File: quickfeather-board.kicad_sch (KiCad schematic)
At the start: 101 parts, among them IC1 EOSAI-S-PUN64, J1 PinHeader_1x2_P2.54mm_Drill1.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, J2 PinHeader_1x12_P2.54m_Drill1.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, J3 61301611121, J4 S2B-PH-SM4-TB(LF)(SN), J5 USB-Micro-B_Molex_473460001, J6 PinHeader_2x5_P1.27mm_SMD_Lat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, J7 PinHeader_1x2_P2.54mm_Drill1.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, J8 PinHeader_2x8_P2.54mm_Drill1mm, Q1 NX3008CBKV, Q2 2N7002PV, Q3 2N7002PV, Q4 DMG1012T-7, U1 TPS62821DLCR, U2 MCP73831T-2AC_SOT, U3 GD25Q16CWIGR, U4 DPS310, U5 MC3635, X1 Resonator_12MHz_445

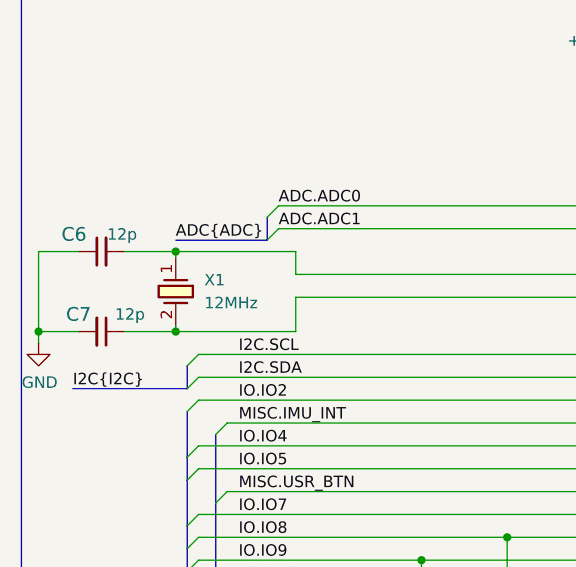
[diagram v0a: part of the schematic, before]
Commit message: [#54927] Update X1
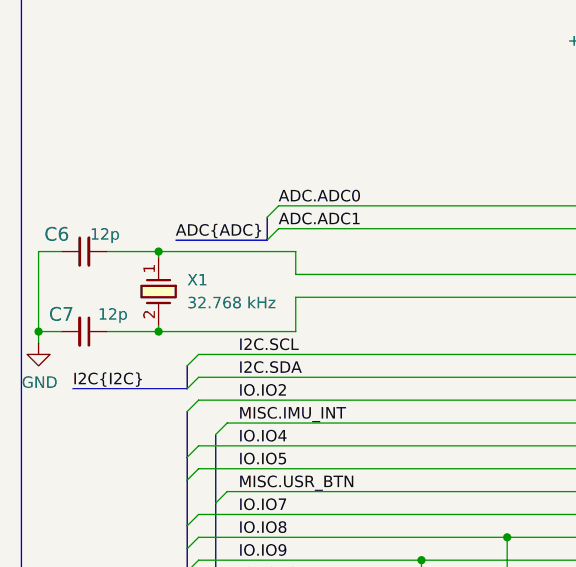
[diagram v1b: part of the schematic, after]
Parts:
- X1: value Resonator_12MHz_445 -> Resonator_32.768kHz_ECX-31B; footprint antmicro-footprints:Resonator_SMD_CTS_445_5x3.2mm -> antmicro-footprints:SMD-2_3.2x1.5mm; symbol antmicroResonators:Resonator_12MHz_445 -> antmicroResonators:Resonator_32.768kHz_ECX-31B; MPN 445I23D12M00000 -> ECS-.327-12.5-34B-TR; Manufacturer CTS -> ECS Inc. International; Val 12MHz -> 32.768 kHz
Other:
- moved on the sheet: C6, C7, X1
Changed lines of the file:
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@@
   (junction (at 356.87 130.81) (diameter 0) (color 0 0 0 0)
   )
+  (junction (at 29.21 44.45) (diameter 0) (color 0 0 0 0)
+  )
   (junction (at 396.875 172.085) (diameter 0) (color 0 0 0 0)
   )
@@
   (junction (at 328.93 34.29) (diameter 0) (color 0 0 0 0)
   )
-  (junction (at 31.115 53.34) (diameter 0) (color 0 0 0 0)
-  )
   (junction (at 76.2 124.46) (diameter 0) (color 0 0 0 0)
   )
+  (junction (at 29.21 53.34) (diameter 0) (color 0 0 0 0)
+  )
   (junction (at 15.875 53.34) (diameter 0) (color 0 0 0 0)
   )
@@
   (junction (at 52.705 220.98) (diameter 0) (color 0 0 0 0)
   )
-  (junction (at 31.115 44.45) (diameter 0) (color 0 0 0 0)
-  )
   (junction (at 194.945 158.115) (diameter 0) (color 0 0 0 0)
   )
@@
     (stroke (width 0) (type default))
   )
-  (wire (pts (xy 25.4 53.34) (xy 31.115 53.34))
+  (wire (pts (xy 23.495 53.34) (xy 29.21 53.34))
     (stroke (width 0) (type default))
   )
@@
     (stroke (width 0) (type default))
   )
+  (wire (pts (xy 29.21 53.34) (xy 44.45 53.34))
+    (stroke (width 0) (type default))
+  )
   (wire (pts (xy 178.435 156.21) (xy 178.435 162.56))
     (stroke (width 0) (type default))
@@
     (stroke (width 0) (type default))
   )
-  (wire (pts (xy 15.875 53.34) (xy 20.32 53.34))
+  (wire (pts (xy 15.875 53.34) (xy 18.415 53.34))
     (stroke (width 0) (type default))
   )
@@
     (stroke (width 0) (type default))
   )
-  (wire (pts (xy 15.875 44.45) (xy 20.32 44.45))
+  (wire (pts (xy 15.875 44.45) (xy 18.415 44.45))
     (stroke (width 0) (type default))
   )
@@
     (stroke (width 0) (type default))
   )
-  (wire (pts (xy 31.115 44.45) (xy 44.45 44.45))
+  (wire (pts (xy 29.21 44.45) (xy 44.45 44.45))
     (stroke (width 0) (type default))
   )
@@
     (stroke (width 0) (type default))
   )
-  (wire (pts (xy 25.4 44.45) (xy 31.115 44.45))
+  (wire (pts (xy 23.495 44.45) (xy 29.21 44.45))
     (stroke (width 0) (type default))
   )
@@
     (stroke (width 0) (type default))
   )
-  (wire (pts (xy 31.115 53.34) (xy 31.115 52.705))
+  (wire (pts (xy 29.21 53.34) (xy 29.21 52.705))
     (stroke (width 0) (type default))
   )
@@
     (stroke (width 0) (type default))
   )
-  (wire (pts (xy 31.115 45.085) (xy 31.115 44.45))
+  (wire (pts (xy 29.21 45.085) (xy 29.21 44.45))
     (stroke (width 0) (type default))
   )
@@
     (stroke (width 0) (type default))
   )
-  (wire (pts (xy 44.45 53.34) (xy 31.115 53.34))
-    (stroke (width 0) (type default))
-  )
   (wire (pts (xy 234.315 221.615) (xy 234.315 231.14))
     (stroke (width 0) (type default))
@@
     )
   )
-  (symbol (lib_id "antmicroResonators:Resonator_12MHz_445") (at 31.115 45.085 270) (unit 1)
+  (symbol (lib_id "antmicroResonators:Resonator_32.768kHz_ECX-31B") (at 29.21 45.085 270) (unit 1)
     (in_bom yes) (on_board yes) (dnp no) (fields_autoplaced)
-    (property "Reference" "X1" (at 34.29 47.625 90)
+    (property "Reference" "X1" (at 32.385 47.625 90)
       (effects (font (size 1.27 1.27)) (justify left))
     )
-    (property "Value" "Resonator_12MHz_445" (at 15.875 60.325 0)
+    (property "Value" "Resonator_32.768kHz_ECX-31B" (at 13.97 60.325 0)
       (effects (font (size 1.27 1.27) (thickness 0.15)) (justify left bottom) hide)
     )
-    (property "Footprint" "antmicro-footprints:Resonator_SMD_CTS_445_5x3.2mm" (at 13.335 60.325 0)
+    (property "Footprint" "antmicro-footprints:SMD-2_3.2x1.5mm" (at 11.43 60.325 0)
       (effects (font (size 1.27 1.27) (thickness 0.15)) (justify left bottom) hide)
     )
-    (property "Datasheet" "https://www.ctscorp.com/wp-content/uploads/445.pdf" (at 10.795 60.325 0)
+    (property "Datasheet" "http://www.ecsxtal.com/store/pdf/ecx-31b.pdf" (at 8.89 60.325 0)
       (effects (font (size 1.27 1.27) (thickness 0.15)) (justify left bottom) hide)
     )
-    (property "MPN" "445I23D12M00000" (at 34.925 48.895 90)
-      (effects (font (size 1.27 1.27) (thickness 0.15)) (justify left) hide)
+    (property "MPN" "ECS-.327-12.5-34B-TR" (at 21.59 60.325 0)
+      (effects (font (size 1.27 1.27) (thickness 0.15)) (justify left bottom) hide)
     )
-    (property "Manufacturer" "CTS" (at 20.955 60.325 0)
+    (property "Manufacturer" "ECS Inc. International" (at 19.05 60.325 0)
       (effects (font (size 1.27 1.27) (thickness 0.15)) (justify left bottom) hide)
     )
-    (property "Val" "12MHz" (at 34.29 50.165 90)
+    (property "Val" "32.768 kHz" (at 32.385 50.165 90)
       (effects (font (size 1.27 1.27) (thickness 0.15)) (justify left))
     )
-    (property "Author" "Antmicro" (at 8.255 60.325 0)
+    (property "Author" "Antmicro" (at 6.35 60.325 0)
       (effects (font (size 1.27 1.27) (thickness 0.15)) (justify left bottom) hide)
     )
-    (property "License" "Apache-2.0" (at 5.715 60.325 0)
+    (property "License" "Apache-2.0" (at 3.81 60.325 0)
       (effects (font (size 1.27 1.27) (thickness 0.15)) (justify left bottom) hide)
     )
@@
     )
   )
-  (symbol (lib_id "antmicroCapacitors0402:C_12p_0402") (at 20.32 44.45 0) (unit 1)
+  (symbol (lib_id "antmicroCapacitors0402:C_12p_0402") (at 18.415 44.45 0) (unit 1)
     (in_bom yes) (on_board yes) (dnp no)
-    (property "Reference" "C6" (at 18.415 42.545 0)
+    (property "Reference" "C6" (at 16.51 42.545 0)
       (effects (font (size 1.524 1.524)) (justify left))
     )
-    (property "Value" "C_12p_0402" (at 20.32 48.26 0)
+    (property "Value" "C_12p_0402" (at 18.415 48.26 0)
       (effects (font (size 1.524 1.524)) hide)
     )
-    (property "Footprint" "antmicro-footprints:C_0402_1005Metric" (at 25.4 39.37 0)
+    (property "Footprint" "antmicro-footprints:C_0402_1005Metric" (at 23.495 39.37 0)
       (effects (font (size 1.524 1.524)) (justify left) hide)
     )
-    (property "Datasheet" "https://product.tdk.com/en/search/capacitor/ceramic/mlcc/info?part_no=CGA2B2C0G1H120J050BA" (at 20.32 44.45 0)
+    (property "Datasheet" "https://product.tdk.com/en/search/capacitor/ceramic/mlcc/info?part_no=CGA2B2C0G1H120J050BA" (at 18.415 44.45 0)
       (effects (font (size 1.27 1.27)) hide)
     )
-    (property "Manufacturer" "TDK" (at 25.4 34.29 0)
+    (property "Manufacturer" "TDK" (at 23.495 34.29 0)
       (effects (font (size 1.524 1.524)) (justify left) hide)
     )
-    (property "MPN" "CGA2B2C0G1H120J050BA" (at 25.4 36.83 0)
+    (property "MPN" "CGA2B2C0G1H120J050BA" (at 23.495 36.83 0)
       (effects (font (size 1.524 1.524)) (justify left) hide)
     )
-    (property "Val" "12p" (at 23.495 42.545 0)
+    (property "Val" "12p" (at 21.59 42.545 0)
       (effects (font (size 1.27 1.27)) (justify left))
     )
-    (property "License" "Apache-2.0" (at 40.64 67.31 0)
+    (property "License" "Apache-2.0" (at 38.735 67.31 0)
       (effects (font (size 1.27 1.27) (thickness 0.15)) (justify left bottom) hide)
     )
-    (property "Author" "Antmicro" (at 40.64 69.85 0)
+    (property "Author" "Antmicro" (at 38.735 69.85 0)
       (effects (font (size 1.27 1.27) (thickness 0.15)) (justify left bottom) hide)
     )
-    (property "Voltage" "" (at 40.64 72.39 0)
+    (property "Voltage" "" (at 38.735 72.39 0)
       (effects (font (size 1.27 1.27)) (justify left bottom) hide)
     )
-    (property "Dielectric" "" (at 40.64 74.93 0)
+    (property "Dielectric" "" (at 38.735 74.93 0)
       (effects (font (size 1.27 1.27)) (justify left bottom) hide)
     )
@@
     )
   )
-  (symbol (lib_id "antmicroCapacitors0402:C_12p_0402") (at 25.4 53.34 180) (unit 1)
+  (symbol (lib_id "antmicroCapacitors0402:C_12p_0402") (at 23.495 53.34 180) (unit 1)
     (in_bom yes) (on_board yes) (dnp no)
-    (property "Reference" "C7" (at 20.32 51.435 0)
+    (property "Reference" "C7" (at 18.415 51.435 0)
       (effects (font (size 1.524 1.524)))
     )
-    (property "Value" "C_12p_0402" (at 25.4 49.53 0)
+    (property "Value" "C_12p_0402" (at 23.495 49.53 0)
       (effects (font (size 1.524 1.524)) hide)
     )
-    (property "Footprint" "antmicro-footprints:C_0402_1005Metric" (at 20.32 58.42 0)
+    (property "Footprint" "antmicro-footprints:C_0402_1005Metric" (at 18.415 58.42 0)
       (effects (font (size 1.524 1.524)) (justify left) hide)
     )
-    (property "Datasheet" "https://product.tdk.com/en/search/capacitor/ceramic/mlcc/info?part_no=CGA2B2C0G1H120J050BA" (at 25.4 53.34 0)
+    (property "Datasheet" "https://product.tdk.com/en/search/capacitor/ceramic/mlcc/info?part_no=CGA2B2C0G1H120J050BA" (at 23.495 53.34 0)
       (effects (font (size 1.27 1.27)) hide)
     )
-    (property "Manufacturer" "TDK" (at 20.32 63.5 0)
+    (property "Manufacturer" "TDK" (at 18.415 63.5 0)
       (effects (font (size 1.524 1.524)) (justify left) hide)
     )
-    (property "MPN" "CGA2B2C0G1H120J050BA" (at 20.32 60.96 0)
+    (property "MPN" "CGA2B2C0G1H120J050BA" (at 18.415 60.96 0)
       (effects (font (size 1.524 1.524)) (justify left) hide)
     )
-    (property "Val" "12p" (at 26.035 51.435 0)
+    (property "Val" "12p" (at 24.13 51.435 0)
       (effects (font (size 1.27 1.27)))
     )
-    (property "License" "Apache-2.0" (at 5.08 30.48 0)
+    (property "License" "Apache-2.0" (at 3.175 30.48 0)
       (effects (font (size 1.27 1.27) (thickness 0.15)) (justify left bottom) hide)
     )
-    (property "Author" "Antmicro" (at 5.08 27.94 0)
+    (property "Author" "Antmicro" (at 3.175 27.94 0)
       (effects (font (size 1.27 1.27) (thickness 0.15)) (justify left bottom) hide)
     )
-    (property "Voltage" "" (at 5.08 25.4 0)
+    (property "Voltage" "" (at 3.175 25.4 0)
       (effects (font (size 1.27 1.27)) (justify left bottom) hide)
     )
-    (property "Dielectric" "" (at 5.08 22.86 0)
+    (property "Dielectric" "" (at 3.175 22.86 0)
       (effects (font (size 1.27 1.27)) (justify left bottom) hide)
     )
